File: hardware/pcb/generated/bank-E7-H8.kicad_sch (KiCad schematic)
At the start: 34 parts, among them U58 SK9822-EC20, U59 SK9822-EC20, U60 SK9822-EC20, U61 SK9822-EC20, U62 SK9822-EC20, U63 SK9822-EC20, U64 SK9822-EC20, U65 SK9822-EC20, U73 TCA9554DWR

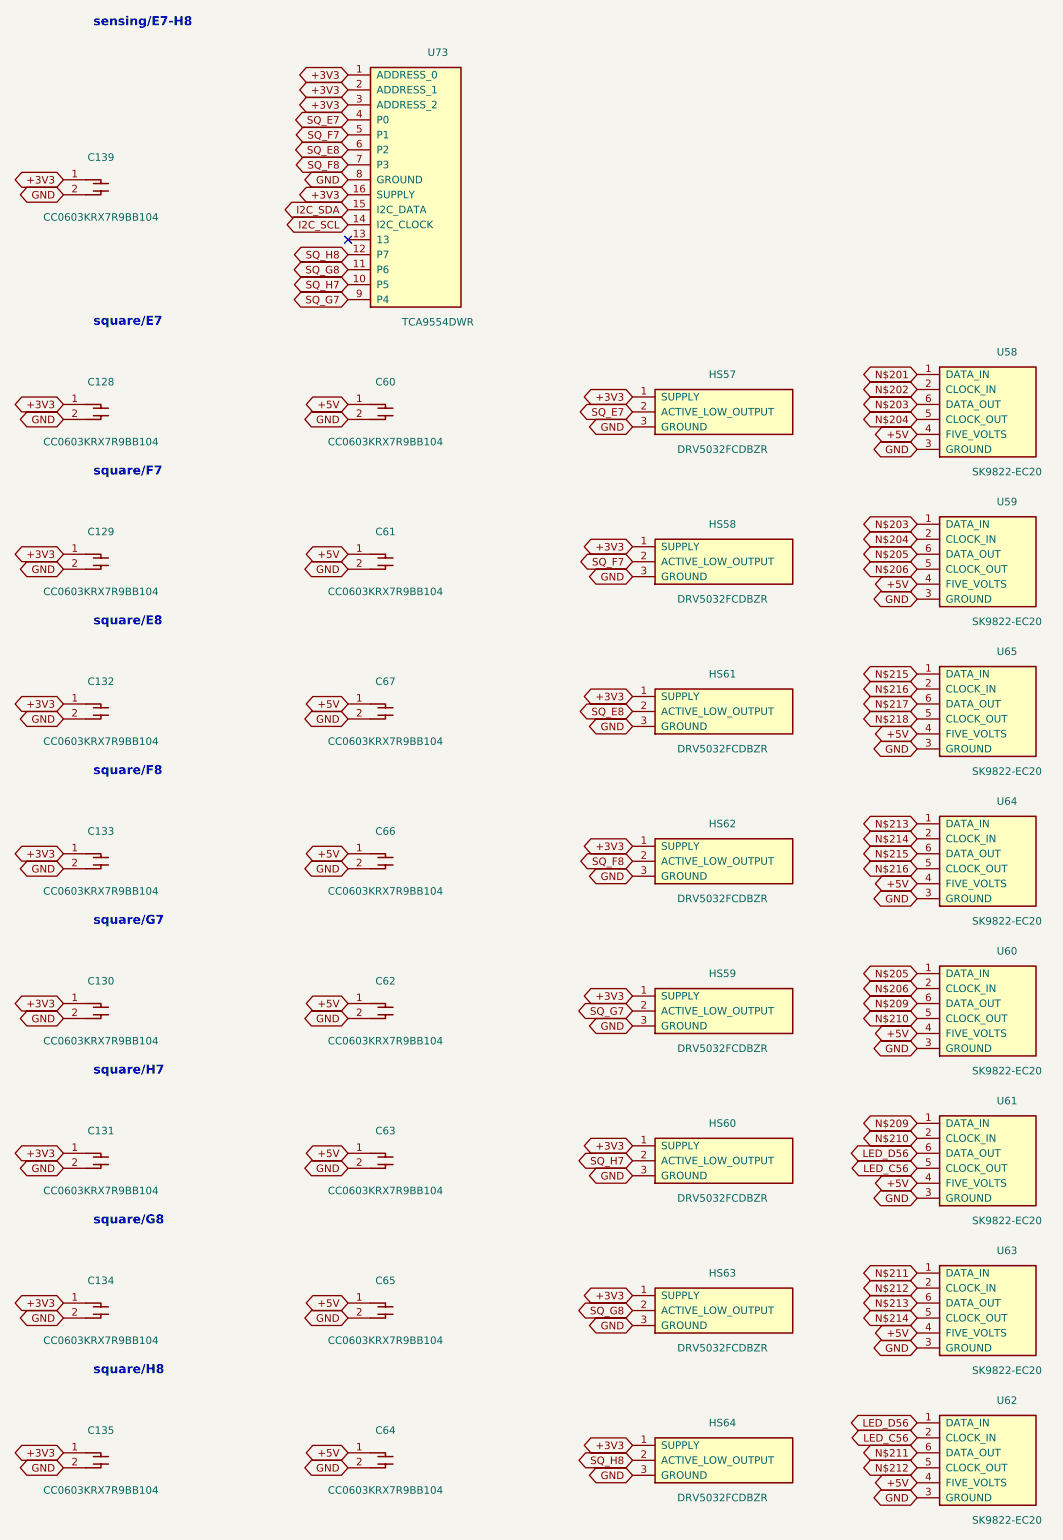
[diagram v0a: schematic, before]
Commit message: chore(pcb): regenerate KiCad, SPICE and review output
Generated by `just pcb` from the committed definition; not hand-edited.
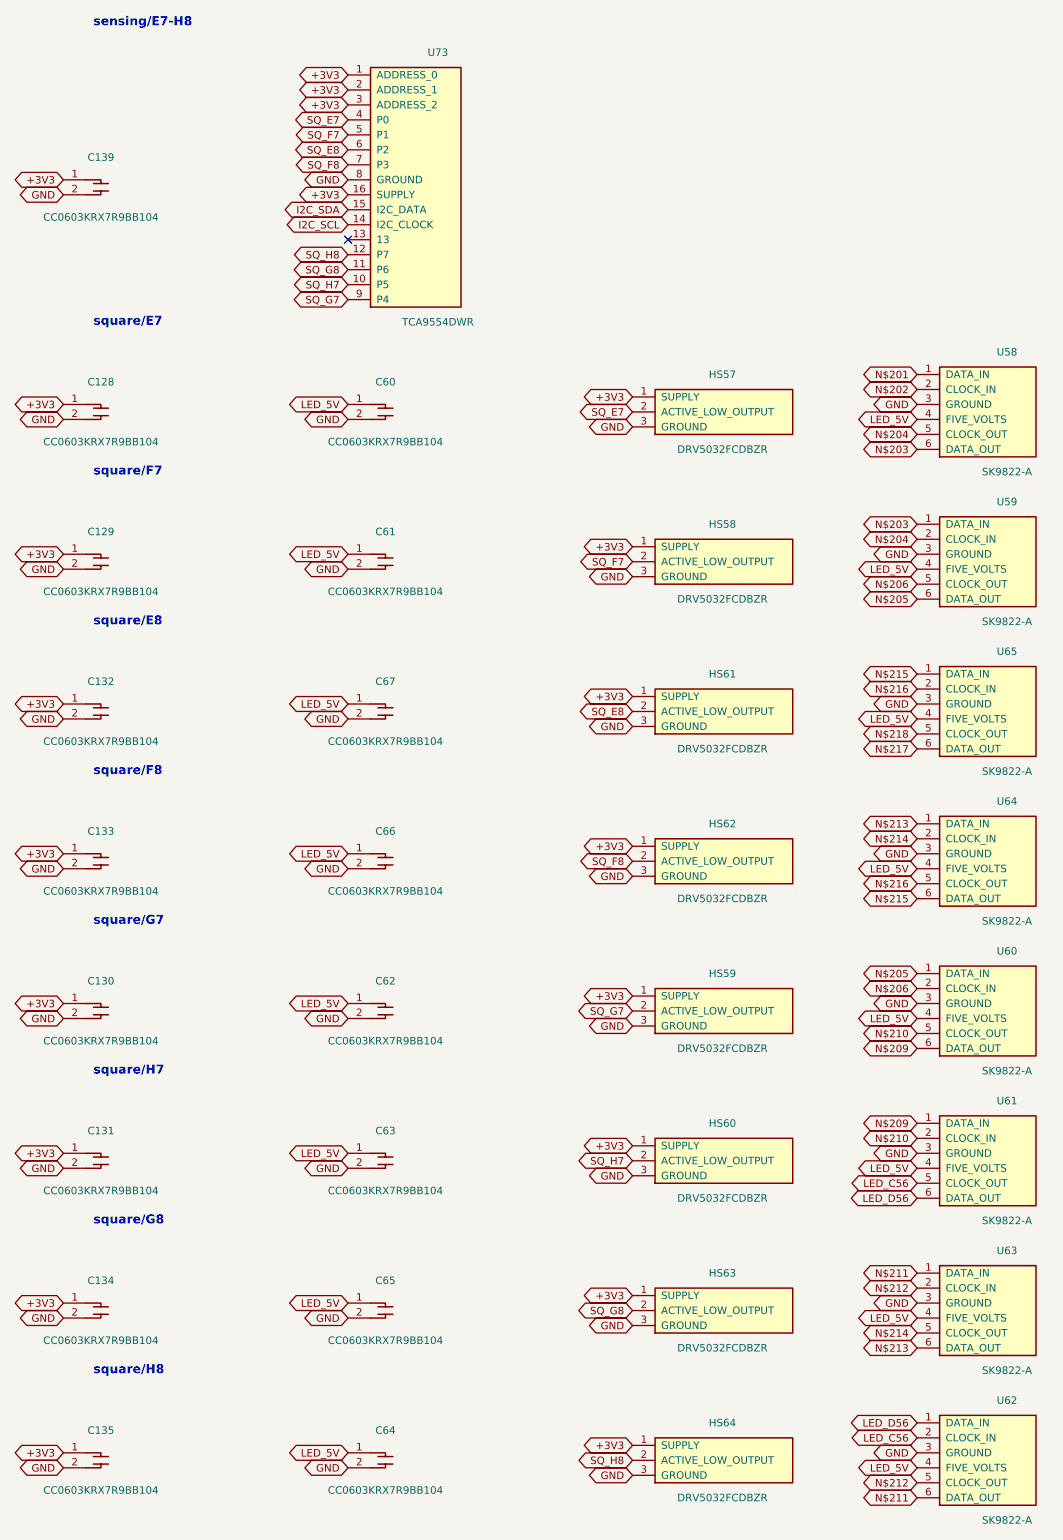
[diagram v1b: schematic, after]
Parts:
- U58, U59, U60, U61, U62, U63, U64, U65: value SK9822-EC20 -> SK9822-A
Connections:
- net +5V renamed LED_5V
